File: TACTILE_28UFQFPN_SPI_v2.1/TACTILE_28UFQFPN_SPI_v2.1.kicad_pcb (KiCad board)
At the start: 2 copper layers, 20 x 32 mm, 16 parts, among them J1 59453-061110ECHLF, J2 59453-061110ECHLF, J3 n.m., U1 STM32G071G8U6N, U2 DRV5056A4, U3 DRV5056A4, U4 DRV5056A4, U5 DRV5056A4

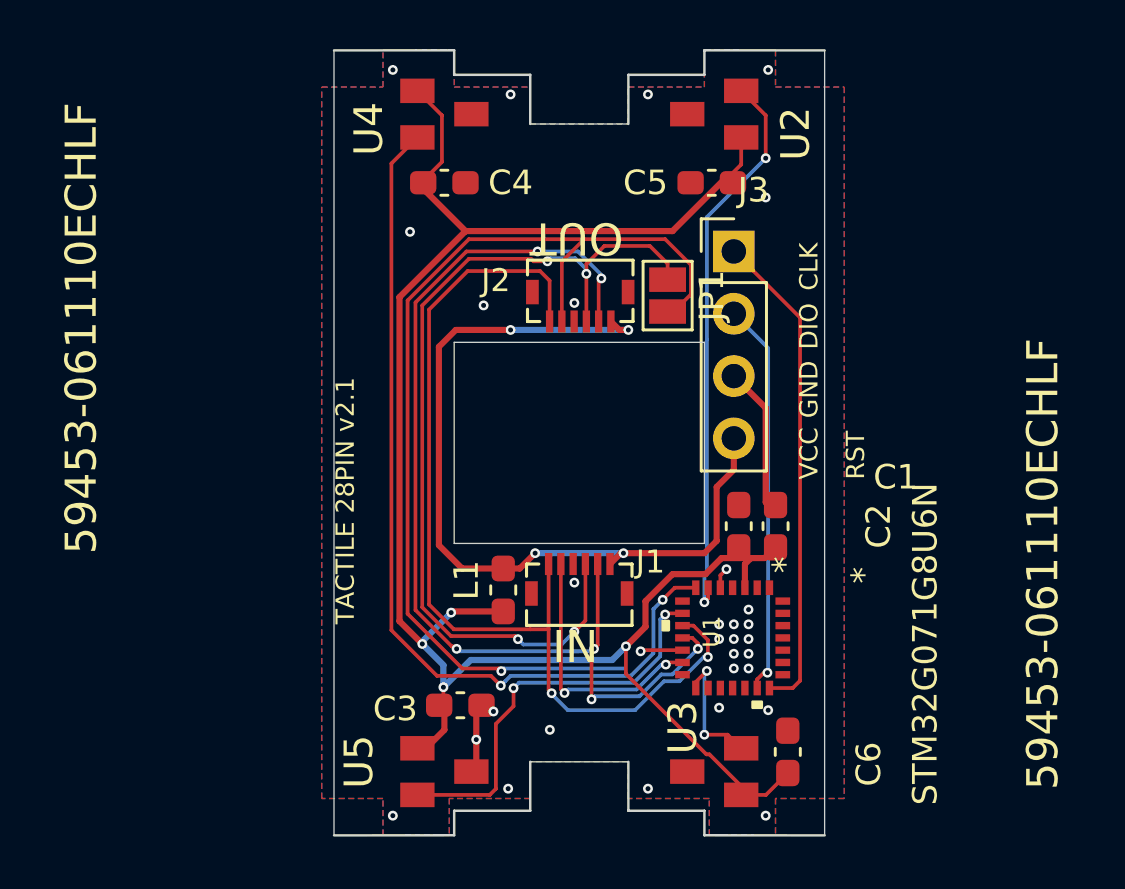
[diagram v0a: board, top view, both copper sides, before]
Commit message: MASTER UPDATE v2
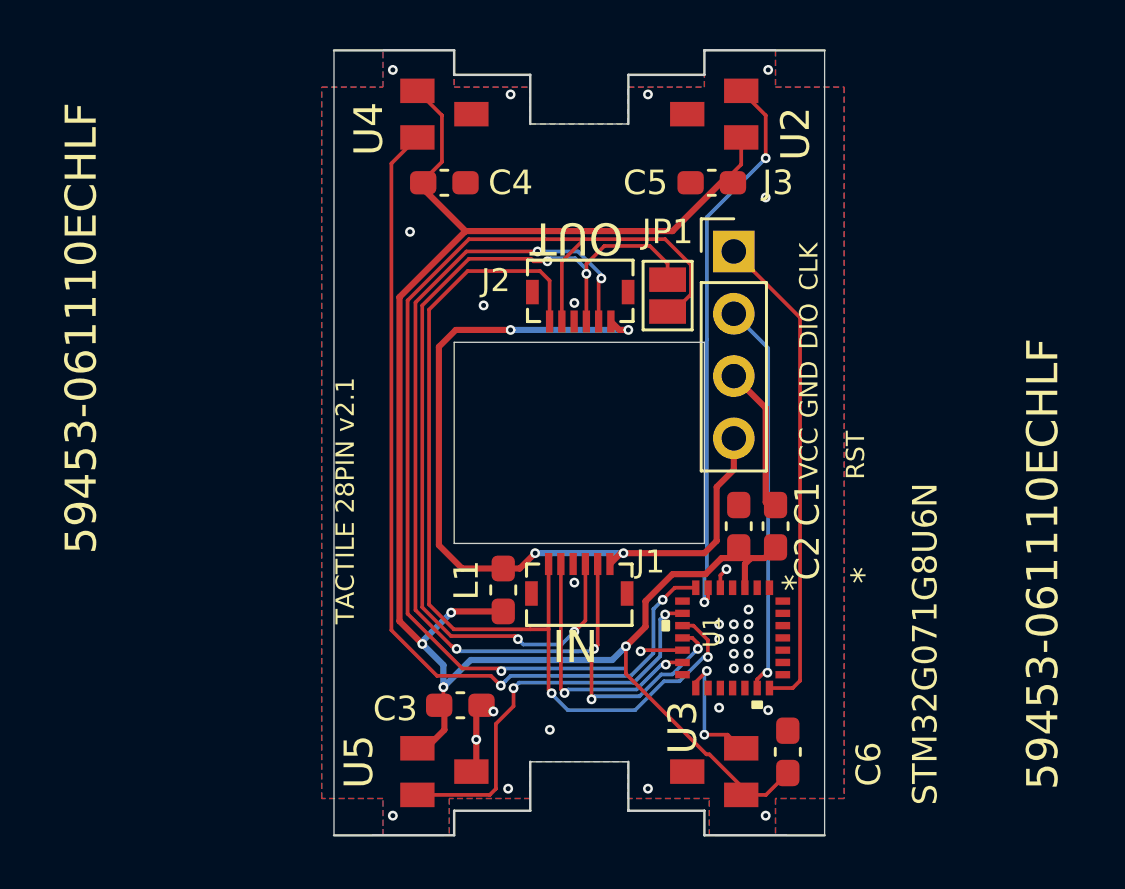
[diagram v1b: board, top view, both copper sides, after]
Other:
- board text added: "GRUBOŚĆ PCB = 0,6mm"
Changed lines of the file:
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@@
     (property "Sheetname" "")
     (attr smd)
-    (fp_text reference "C1" (at 2 6.4 180) (layer "F.SilkS")
+    (fp_text reference "C1" (at 0.9 2.8 270) (layer "F.SilkS")
       (effects (font (size 1 1) (thickness 0.15)))
     )
@@
     (property "Sheetname" "")
     (attr exclude_from_pos_files exclude_from_bom)
-    (fp_text reference "JP1" (at 0 -1.8 -90) (layer "F.SilkS")
+    (fp_text reference "JP1" (at -2.6 0) (layer "F.SilkS")
       (effects (font (size 1 1) (thickness 0.15)))
     )
@@
     (property "Sheetname" "")
     (attr through_hole)
-    (fp_text reference "J3" (at 0.8 -2.5) (layer "F.SilkS")
+    (fp_text reference "J3" (at 1.8 -2.8) (layer "F.SilkS")
       (effects (font (size 1 1) (thickness 0.15)))
     )
@@
       (effects (font (size 1 1) (thickness 0.15)))
     )
-    (fp_text user "*" (at -2.979674 -2.13233 -90) (layer "F.SilkS")
+    (fp_text user "*" (at -2.2536 -2.5489 -90) (layer "F.SilkS")
       (effects (font (size 1 1) (thickness 0.15)))
     )
@@
     (property "Sheetname" "")
     (attr smd)
-    (fp_text reference "C2" (at 0 4.2 90) (layer "F.SilkS")
+    (fp_text reference "C2" (at -1.3 1.3 90) (layer "F.SilkS")
       (effects (font (size 1 1) (thickness 0.15)))
     )
@@
     (fp_line (start -0.8 0.4) (end -0.8 -0.4) (layer "F.Fab") (width 0.1))
     (pad "1" smd roundrect locked (at -0.8625 0 90) (size 1.075 0.95) (layers "F.Cu" "F.Paste" "F.Mask") (roundrect_rratio 0.25)
-      (net 1 "VCC") (pinfunction "1") (pintype "passive"))
+      (net 1 "VCC") (pinfunction "1"))
     (pad "2" smd roundrect locked (at 0.8625 0 90) (size 1.075 0.95) (layers "F.Cu" "F.Paste" "F.Mask") (roundrect_rratio 0.25)
-      (net 2 "GND") (pinfunction "2") (pintype "passive"))
+      (net 2 "GND") (pinfunction "2"))
     (model "${KIPRJMOD}/../common_libraries/3dmodels/C_0603_1608Metric.step"
       (offset (xyz 0 0 0))
@@
     (effects (font (size 0.747776 0.747776) (thickness 0.065024)) (justify left bottom))
   )
+  (gr_text "GRUBOŚĆ PCB = 0,6mm" (at 139.7 131.4) (layer "Cmts.User")
+    (effects (font (size 5 5) (thickness 0.3)))
+  )
   (segment (start 153.803811 117.700889) (end 155.1011 118.998178) (width 0.1524) (layer "F.Cu") (net 1))
